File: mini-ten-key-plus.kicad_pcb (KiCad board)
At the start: 2 copper layers, 95.2 x 95.2 mm, 64 parts, among them SW0 SW_Push, U0 ProMicro

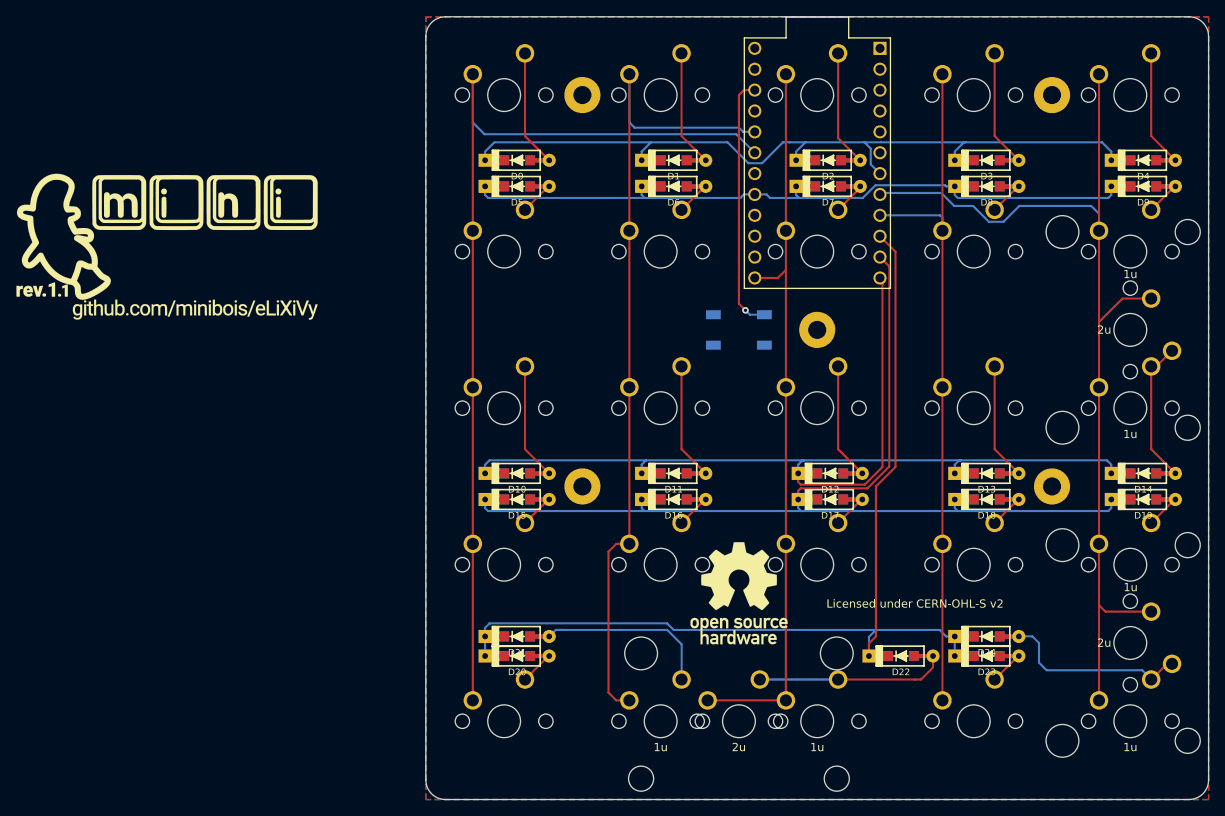
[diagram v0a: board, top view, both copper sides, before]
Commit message: Made gerber files
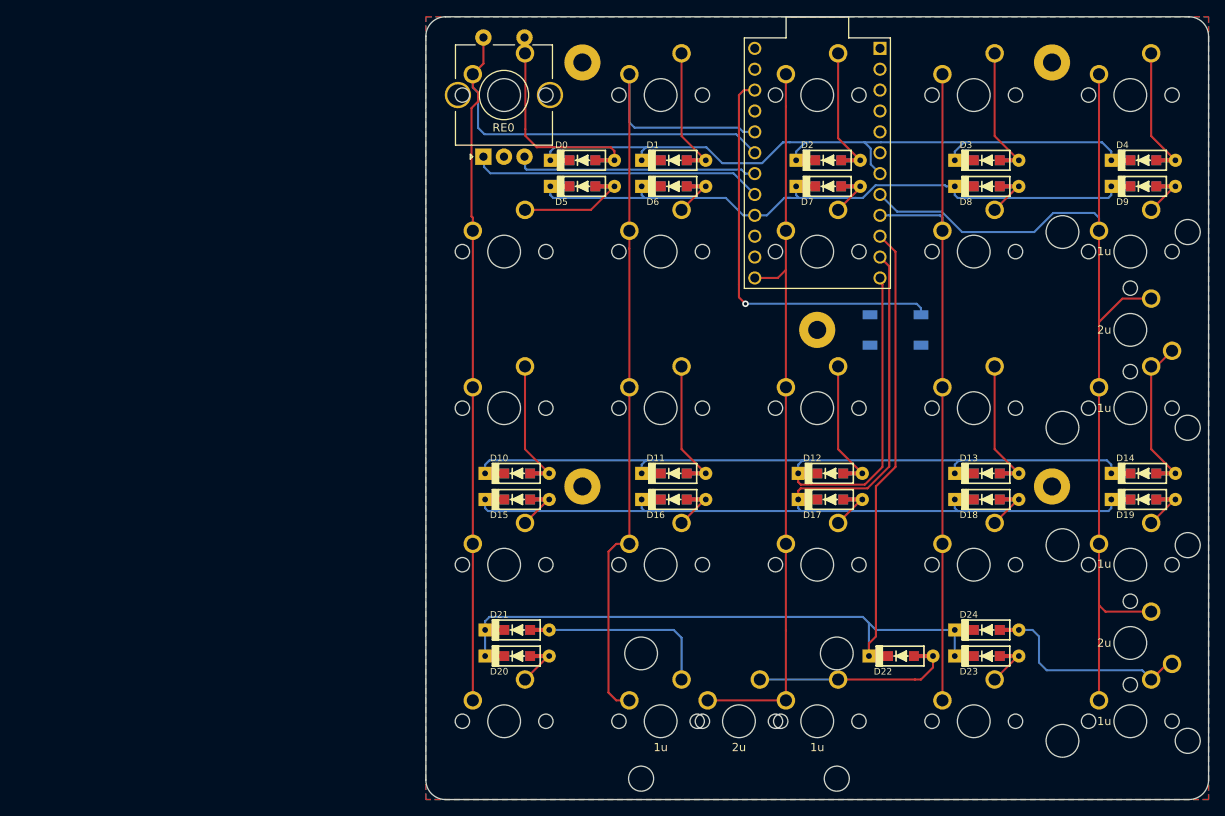
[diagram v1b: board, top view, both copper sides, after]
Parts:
- added RE0: Rotary_Encoder_Switch, mini-general-tweaks:RotaryEncoder_Alps_EC11E-Switch-Vertical-EDIT, F.Cu at (195.1, 86.1)
- LO0: footprint mini-Logos:eLiXiVy-rev1.1-SilkScreen -> mini-Logos:mini-TKP-BSilk
- LO1: footprint mini-Logos:eLiXiVy-rev1.1-Mask -> mini-Logos:mini-TKP-BMask
- LO2: moved to B.Cu
- moved LO0 56.9 mm to (213.0, 105.2)
- moved LO1 56.9 mm to (213.0, 105.2)
- moved RESET 19.1 mm to (245.3, 107.2)
- moved D0 7.94 mm to (207.2, 86.5)
- moved D5 7.94 mm to (207.2, 89.7)
- moved H0 3.97 mm to (264.3, 74.6)
- moved H4 3.97 mm to (207.2, 74.6)
- moved D21 0.79 mm to (199.2, 143.7)
- moved D24 0.79 mm to (256.4, 143.7)
- turned LO2 to 180 degrees
- renumbered SW0 to RESET
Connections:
- net Net-(D0-Pad2) renamed ROW0_RE
- U0 pad 16: Net-(U0-Pad16) -> ROW1
- U0 pad 17: ROW1 -> RE+
- U0 pad 18: Net-(U0-Pad18) -> RE-
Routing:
- net RE+: track 0.00 -> 35.6 mm
- net RE-: track 0.00 -> 29.6 mm
- net RESET: track 31.2 -> 50.3 mm
- net ROW0_RE: track 14.2 -> 24.7 mm
- net ROW0: track 94.3 -> 85.0 mm
- net Net-(D5-Pad2): track 4.13 -> 12.1 mm
- net ROW1: track 84.1 -> 78.4 mm
- net COL0: track 117.9 -> 123.6 mm
- net ROW4: track 120.6 -> 122.7 mm
- net Net-(D24-Pad2): track 23.0 -> 23.8 mm
